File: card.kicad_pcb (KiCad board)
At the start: 2 copper layers, 55 x 85 mm, 9 parts, among them CON1 USB-MINI-B, IC1 ATTINY44-S, P1 CONN_3X2

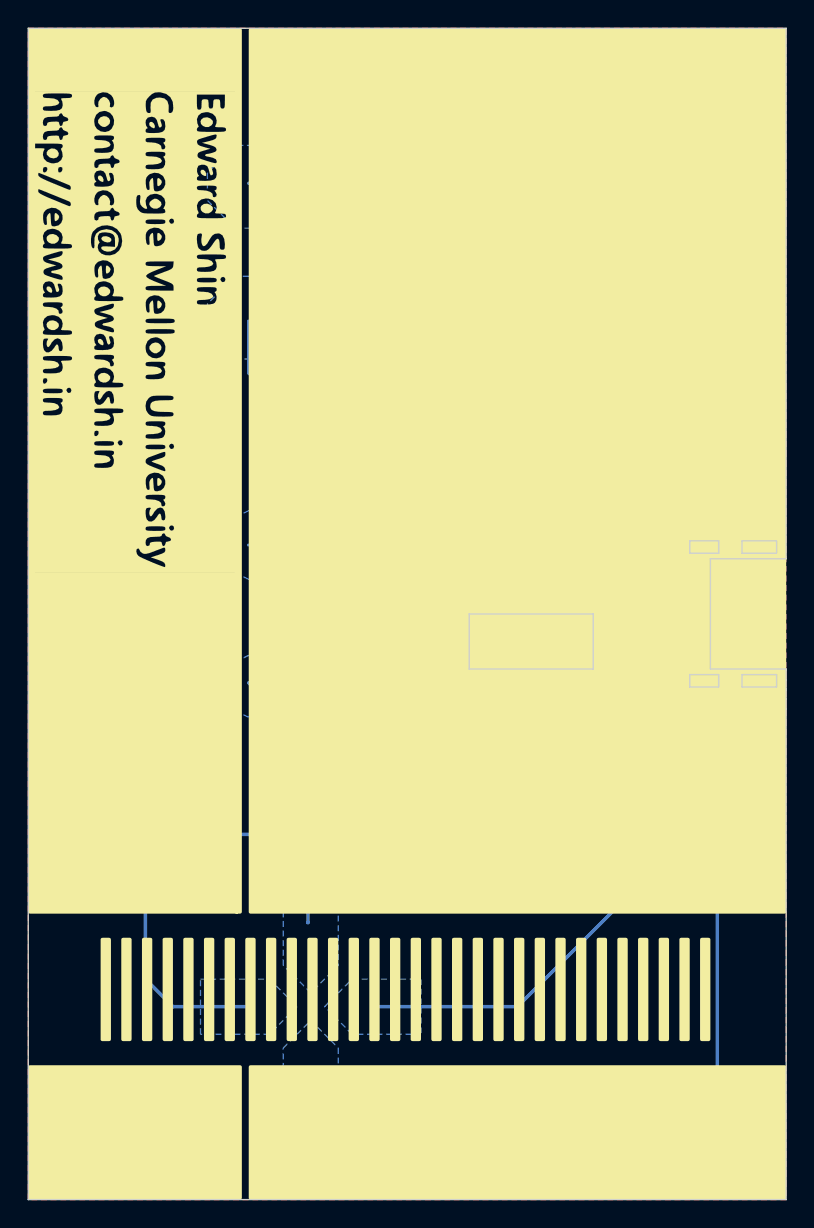
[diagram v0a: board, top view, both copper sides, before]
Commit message: rev C to fab
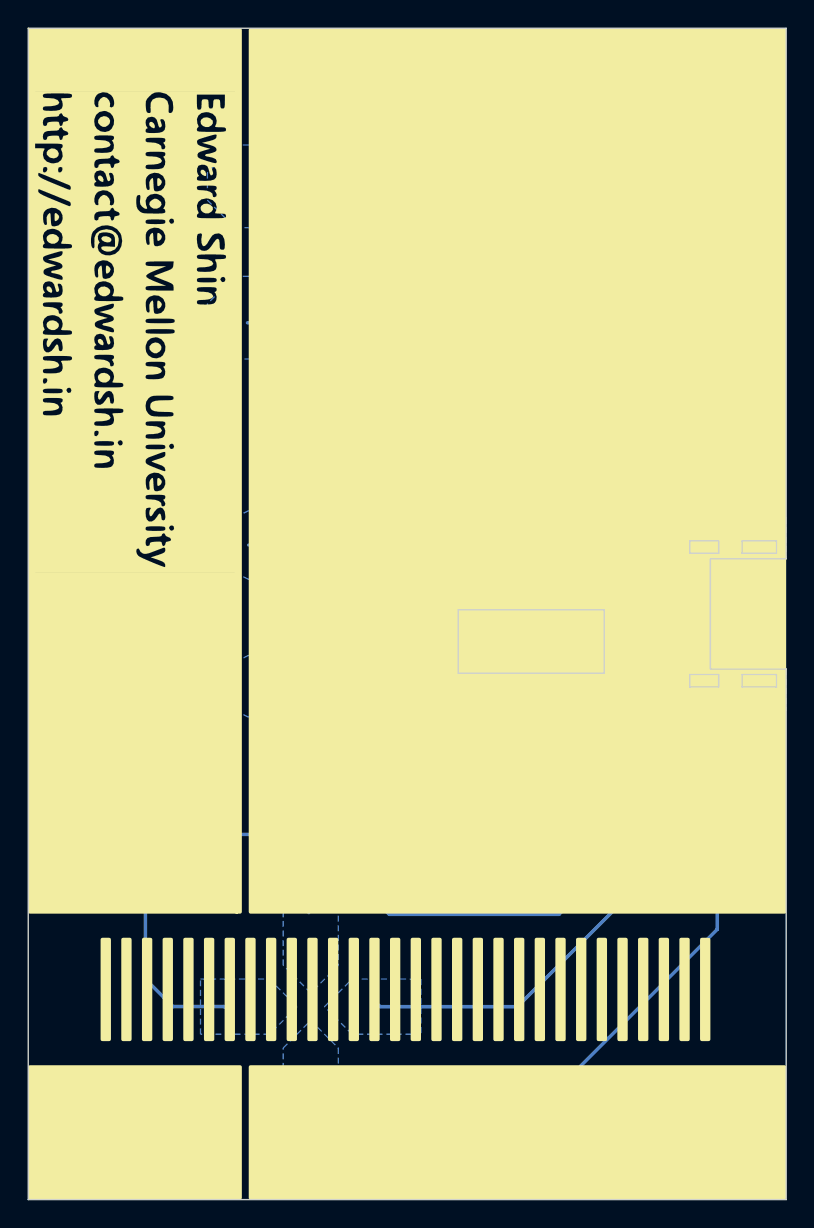
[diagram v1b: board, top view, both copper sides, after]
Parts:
- P1: moved to B.Cu
- moved D1 0.98 mm to (189.5, 88.5), turned to 270 degrees
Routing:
- net +5V: track 32.5 -> 43.7 mm, vias 1 -> 2
- net /MOSI: track 48.8 -> 59.4 mm, vias 1 -> 2
- net (no net): track 265.4 -> 257.0 mm
- net /SCK: track 37.0 -> 29.5 mm, vias 0 -> 2
- net /RST: track 30.9 -> 24.7 mm, vias 1 -> 2
- net GND: track 48.6 -> 52.4 mm, vias 3 -> 4
- net /MISO: track 32.0 -> 28.5 mm
- net N-0000017: track 11.3 -> 12.4 mm
- net N-0000016: track 13.7 -> 12.9 mm
- added copper zone on B.Cu, net (none)
- removed copper zone on F.Cu, net GND
- removed copper zone on B.Cu, net N-000001
- removed copper zone on B.Cu, net N-000002
- removed copper zone on B.Cu, net N-000003
- removed copper zone on B.Cu, net N-000005
- removed copper zone on B.Cu, net N-000006
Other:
- outline, holes or cut-outs redrawn
- board text removed: "CUTOUT"
